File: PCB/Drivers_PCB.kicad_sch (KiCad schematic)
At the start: 30 parts, among them J1 Power_Connector, J10 Conn_01x08, J2 Fan_Connector, J3 Motor_1_connector, J4 EOC_Switch_Connector, J5 Motor_2_connector, J6 IR_LED_Connector, J7 Conn_01x08, J8 Conn_01x06, J9 Conn_01x10, U1 A4988, U2 A4988

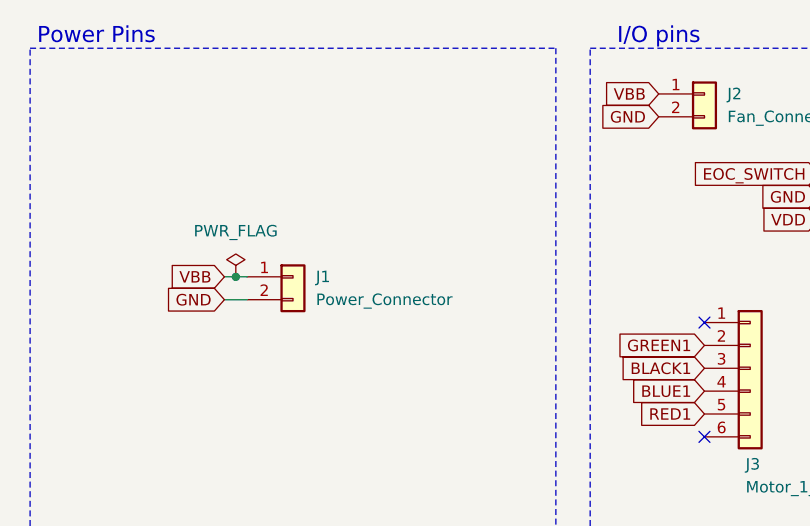
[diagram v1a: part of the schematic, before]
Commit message: Cleaning the git
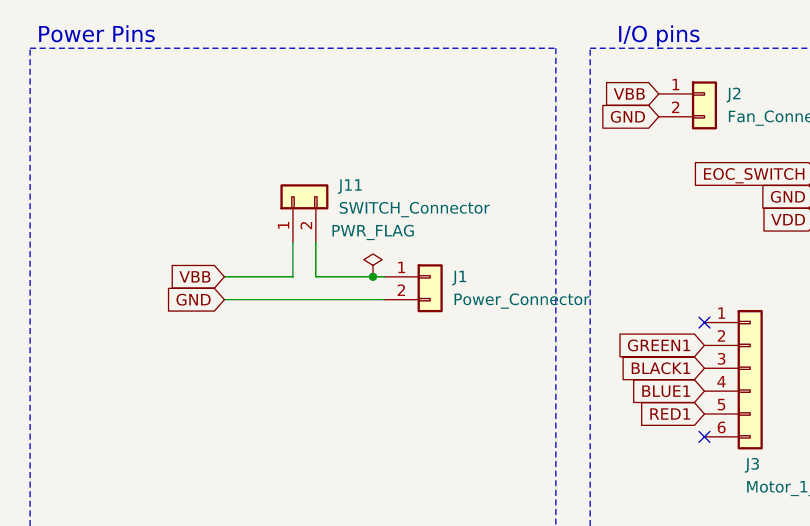
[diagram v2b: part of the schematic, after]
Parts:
- added J11: SWITCH_Connector, Connector_JST:JST_XH_B2B-XH-A_1x02_P2.50mm_Vertical, symbol Connector_Generic:Conn_01x02
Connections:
- net VBB: now also J11.1 (Pin_1); no longer J1.1 (Pin_1)
- new net: J1.1 (Pin_1), J11.2 (Pin_2)
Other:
- moved on the sheet: J1
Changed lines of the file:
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@@
 	)
 	(junction
-		(at 46.99 49.53)
-		(diameter 0)
-		(color 0 0 0 0)
-	)
-	(junction
 		(at 128.27 160.02)
 		(diameter 0)
@@
 	)
 	(junction
+		(at 62.23 49.53)
+		(diameter 0)
+		(color 0 0 0 0)
+	)
+	(junction
 		(at 265.43 114.3)
 		(diameter 0)
@@
 	(wire
 		(pts
-			(xy 168.91 114.3) (xy 168.91 116.84)
+			(xy 62.23 49.53) (xy 63.5 49.53)
 		)
 		(stroke
@@
 	(wire
 		(pts
-			(xy 273.05 142.24) (xy 273.05 127)
+			(xy 168.91 114.3) (xy 168.91 116.84)
 		)
 		(stroke
@@
 	(wire
 		(pts
-			(xy 121.92 160.02) (xy 128.27 160.02)
+			(xy 273.05 142.24) (xy 273.05 127)
 		)
 		(stroke
@@
 	(wire
 		(pts
-			(xy 265.43 118.11) (xy 259.08 118.11)
+			(xy 121.92 160.02) (xy 128.27 160.02)
 		)
 		(stroke
@@
 	(wire
 		(pts
-			(xy 168.91 142.24) (xy 173.99 142.24)
+			(xy 265.43 118.11) (xy 259.08 118.11)
 		)
 		(stroke
@@
 	(wire
 		(pts
-			(xy 154.94 127) (xy 158.75 127)
+			(xy 168.91 142.24) (xy 173.99 142.24)
 		)
 		(stroke
@@
 	(wire
 		(pts
-			(xy 116.84 99.06) (xy 121.92 99.06)
+			(xy 154.94 127) (xy 158.75 127)
 		)
 		(stroke
@@
 	(wire
 		(pts
-			(xy 45.72 49.53) (xy 46.99 49.53)
+			(xy 116.84 99.06) (xy 121.92 99.06)
 		)
 		(stroke
@@
 	(wire
 		(pts
+			(xy 53.34 49.53) (xy 53.34 45.72)
+		)
+		(stroke
+			(width 0)
+			(type default)
+		)
+	)
+	(wire
+		(pts
 			(xy 121.92 99.06) (xy 121.92 101.6)
 		)
@@
 	(wire
 		(pts
+			(xy 55.88 49.53) (xy 62.23 49.53)
+		)
+		(stroke
+			(width 0)
+			(type default)
+		)
+	)
+	(wire
+		(pts
 			(xy 220.98 99.06) (xy 226.06 99.06)
 		)
@@
 	(wire
 		(pts
-			(xy 46.99 49.53) (xy 48.26 49.53)
+			(xy 97.79 114.3) (xy 104.14 114.3)
 		)
 		(stroke
@@
 	(wire
 		(pts
-			(xy 97.79 114.3) (xy 104.14 114.3)
+			(xy 265.43 114.3) (xy 273.05 114.3)
 		)
 		(stroke
@@
 	(wire
 		(pts
-			(xy 265.43 114.3) (xy 273.05 114.3)
+			(xy 128.27 157.48) (xy 128.27 160.02)
 		)
 		(stroke
@@
 	(wire
 		(pts
-			(xy 128.27 157.48) (xy 128.27 160.02)
+			(xy 55.88 45.72) (xy 55.88 49.53)
 		)
 		(stroke
@@
 	(wire
 		(pts
-			(xy 45.72 52.07) (xy 48.26 52.07)
+			(xy 45.72 52.07) (xy 63.5 52.07)
 		)
 		(stroke
@@
 	(wire
 		(pts
+			(xy 45.72 49.53) (xy 53.34 49.53)
+		)
+		(stroke
+			(width 0)
+			(type default)
+		)
+	)
+	(wire
+		(pts
 			(xy 259.08 127) (xy 262.89 127)
 		)
@@
 	(symbol
 		(lib_id "Connector_Generic:Conn_01x02")
-		(at 53.34 49.53 0)
+		(at 68.58 49.53 0)
 		(unit 1)
 		(exclude_from_sim no)
@@
 		(fields_autoplaced yes)
 		(property "Reference" "J1"
-			(at 55.88 49.5299 0)
+			(at 71.12 49.5299 0)
 			(effects
 				(font
@@
 		)
 		(property "Value" "Power_Connector"
-			(at 55.88 52.0699 0)
+			(at 71.12 52.0699 0)
 			(effects
 				(font
@@
 		)
 		(property "Footprint" "TerminalBlock:TerminalBlock_bornier-2_P5.08mm"
-			(at 53.34 49.53 0)
+			(at 68.58 49.53 0)
 			(effects
 				(font
@@
 		)
 		(property "Datasheet" "~"
-			(at 53.34 49.53 0)
+			(at 68.58 49.53 0)
 			(effects
 				(font
@@
 		)
 		(property "Description" "Generic connector, single row, 01x02, script generated (kicad-library-utils/schlib/autogen/connector/)"
-			(at 53.34 49.53 0)
+			(at 68.58 49.53 0)
 			(effects
 				(font
@@
 	(symbol
 		(lib_id "power:PWR_FLAG")
-		(at 46.99 49.53 0)
+		(at 62.23 49.53 0)
 		(unit 1)
 		(exclude_from_sim no)
@@
 		(fields_autoplaced yes)
 		(property "Reference" "#FLG01"
-			(at 46.99 47.625 0)
+			(at 62.23 47.625 0)
 			(effects
 				(font
@@
 		)
 		(property "Value" "PWR_FLAG"
-			(at 46.99 44.45 0)
+			(at 62.23 44.45 0)
 			(effects
 				(font
@@
 		)
 		(property "Footprint" ""
-			(at 46.99 49.53 0)
+			(at 62.23 49.53 0)
 			(effects
 				(font
@@
 		)
 		(property "Datasheet" "~"
-			(at 46.99 49.53 0)
+			(at 62.23 49.53 0)
 			(effects
 				(font
@@
 		)
 		(property "Description" "Special symbol for telling ERC where power comes from"
-			(at 46.99 49.53 0)
+			(at 62.23 49.53 0)
 			(effects
 				(font
@@
 					(unit 1)
 				)
+			)
+		)
+	)
+	(symbol
+		(lib_id "Connector_Generic:Conn_01x02")
+		(at 53.34 40.64 90)
+		(unit 1)
+		(exclude_from_sim no)
+		(in_bom yes)
+		(on_board yes)
+		(dnp no)
+		(fields_autoplaced yes)
+		(property "Reference" "J11"
+			(at 58.42 39.3699 90)
+			(effects
+				(font
+					(size 1.27 1.27)
+				)
+				(justify right)
+			)
+		)
+		(property "Value" "SWITCH_Connector"
+			(at 58.42 41.9099 90)
+			(effects
+				(font
+					(size 1.27 1.27)
+				)
+				(justify right)
+			)
+		)
+		(property "Footprint" "Connector_JST:JST_XH_B2B-XH-A_1x02_P2.50mm_Vertical"
+			(at 53.34 40.64 0)
+			(effects
+				(font
+					(size 1.27 1.27)
+				)
+				(hide yes)
+			)
+		)
+		(property "Datasheet" "~"
+			(at 53.34 40.64 0)
+			(effects
+				(font
+					(size 1.27 1.27)
+				)
+				(hide yes)
+			)
+		)
+		(property "Description" "Generic connector, single row, 01x02, script generated (kicad-library-utils/schlib/autogen/connector/)"
+			(at 53.34 40.64 0)
+			(effects
+				(font
+					(size 1.27 1.27)
+				)
+				(hide yes)
+			)
+		)
+		(pin "1"
+		)
+		(pin "2"
+		)
+		(instances
+			(project "Drivers_PCB"
+				(path "/965d1d26-667e-4a58-b302-d26df24cf4f3"
+					(reference "J11")
+					(unit 1)
+				)
